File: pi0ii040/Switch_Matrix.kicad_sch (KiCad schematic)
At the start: 1 part

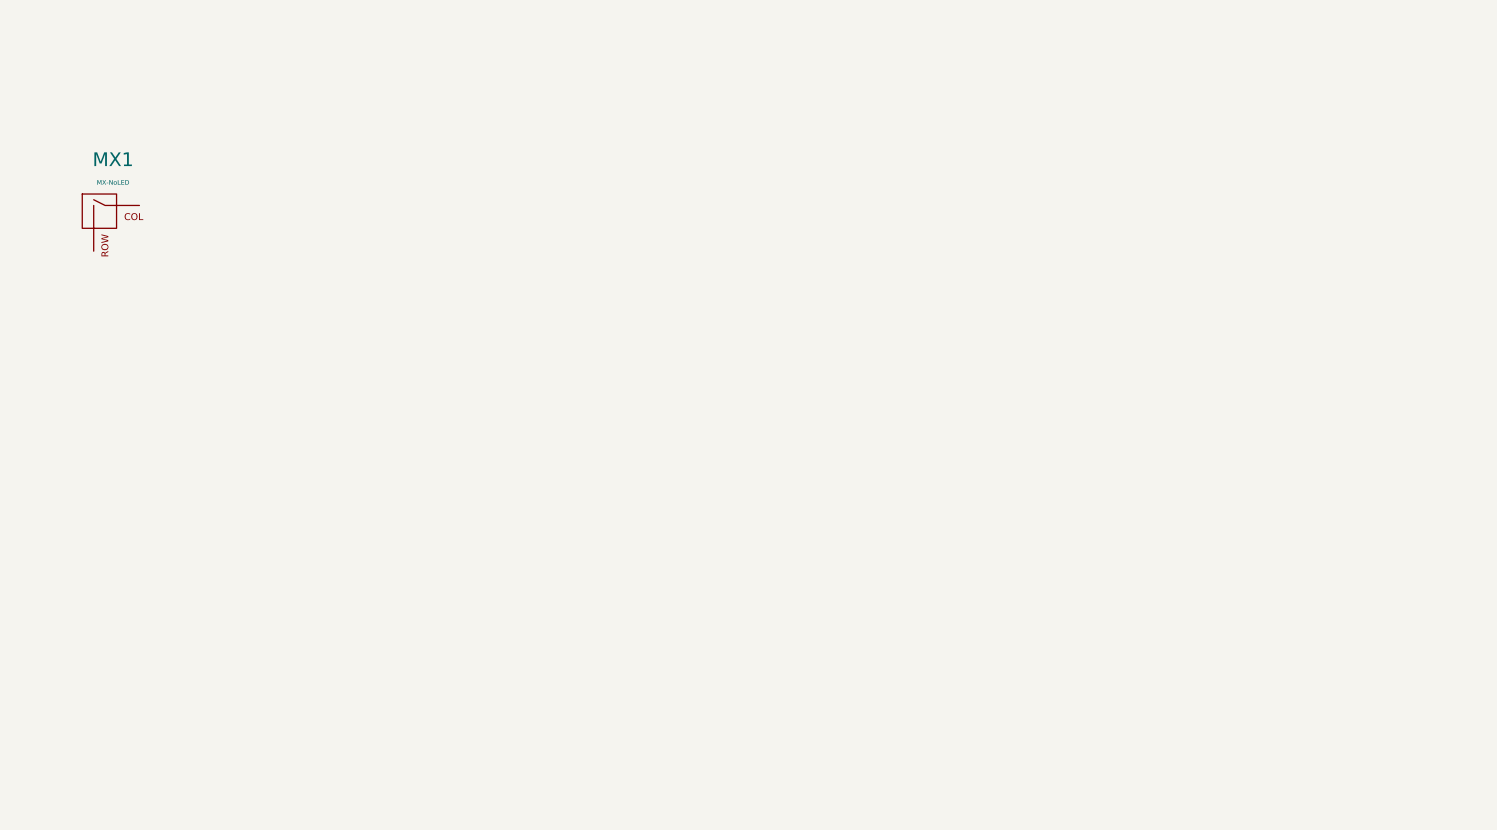
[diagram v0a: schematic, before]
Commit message: Finish? pcb
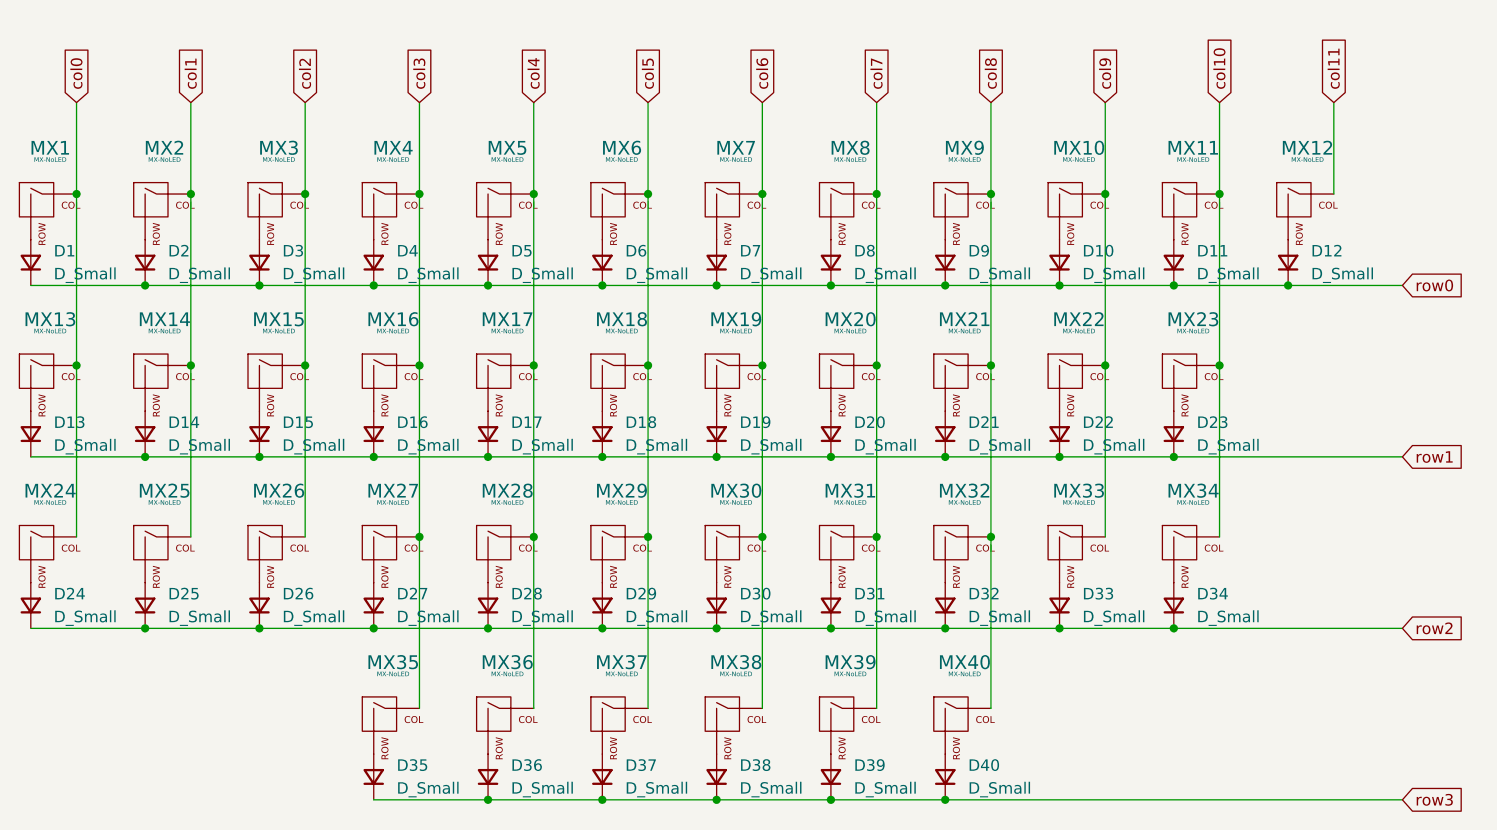
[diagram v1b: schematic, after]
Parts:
- removed MX1: MX-NoLED, symbol MX_Alps_Hybrid:MX-NoLED
- added D1, D10, D11, D12, D13, D14, D15, D16, D17, D18, D19, D2, D20, D21, D22, D23, D24, D25, D26, D27, D28, D29, D3, D30, D31, D32, D33, D34, D35, D36, D37, D38, D39, D4, D40, D5, D6, D7, D8, D9: D_Small, Diode_SMD:D_SOD-123, symbol Device:D_Small
- added MX1, MX10, MX11, MX12, MX14, MX15, MX16, MX17, MX18, MX19, MX2, MX20, MX21, MX22, MX25, MX26, MX27, MX28, MX29, MX3, MX30, MX31, MX32, MX33, MX35, MX4, MX40, MX5, MX6, MX7, MX8, MX9: MX-NoLED, MX_Only:MXOnly-1U-NoLED, symbol cipulot_parts:MX-NoLED
- added MX13, MX34, MX36, MX39: MX-NoLED, MX_Only:MXOnly-1.25U-NoLED, symbol cipulot_parts:MX-NoLED
- added MX23, MX24: MX-NoLED, MX_Only:MXOnly-1.75U-NoLED, symbol cipulot_parts:MX-NoLED
- added MX37: MX-NoLED, MX_Only:MXOnly-2.75U-ReversedStabilizers-NoLED, symbol cipulot_parts:MX-NoLED
- added MX38: MX-NoLED, MX_Only:MXOnly-2.25U-ReversedStabilizers-NoLED, symbol cipulot_parts:MX-NoLED
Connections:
- new net: D21.2 (A), MX21.2 (ROW)
- new net: D10.2 (A), MX10.2 (ROW)
- new net: D40.2 (A), MX40.2 (ROW)
- new net: D16.2 (A), MX16.2 (ROW)
- new net: D28.2 (A), MX28.2 (ROW)
- new net: D39.2 (A), MX39.2 (ROW)
- new net: D23.2 (A), MX23.2 (ROW)
- new net: D1.2 (A), MX1.2 (ROW)
- new net: D27.2 (A), MX27.2 (ROW)
- new net: D32.2 (A), MX32.2 (ROW)
- new net: D31.2 (A), MX31.2 (ROW)
- new net: D13.2 (A), MX13.2 (ROW)
- new net: D11.2 (A), MX11.2 (ROW)
- new net: D18.2 (A), MX18.2 (ROW)
- new net: D25.2 (A), MX25.2 (ROW)
- new net: D14.2 (A), MX14.2 (ROW)
- new net: D8.2 (A), MX8.2 (ROW)
- new net: D22.2 (A), MX22.2 (ROW)
- new net: D26.2 (A), MX26.2 (ROW)
- new net: D34.2 (A), MX34.2 (ROW)
- new net: D19.2 (A), MX19.2 (ROW)
- new net: D12.2 (A), MX12.2 (ROW)
- new net: D15.2 (A), MX15.2 (ROW)
- new net: D4.2 (A), MX4.2 (ROW)
- new net: D5.2 (A), MX5.2 (ROW)
- new net: D24.2 (A), MX24.2 (ROW)
- new net: D30.2 (A), MX30.2 (ROW)
- new net: D37.2 (A), MX37.2 (ROW)
- new net: D17.2 (A), MX17.2 (ROW)
- new net: D35.2 (A), MX35.2 (ROW)
- new net: D20.2 (A), MX20.2 (ROW)
- new net: D3.2 (A), MX3.2 (ROW)
- new net: D6.2 (A), MX6.2 (ROW)
- new net: D38.2 (A), MX38.2 (ROW)
- new net: D29.2 (A), MX29.2 (ROW)
- new net: D2.2 (A), MX2.2 (ROW)
- new net: D33.2 (A), MX33.2 (ROW)
- new net: D9.2 (A), MX9.2 (ROW)
- new net: D7.2 (A), MX7.2 (ROW)
- new net: D36.2 (A), MX36.2 (ROW)
- new net col0: MX1.1 (COL), MX13.1 (COL), MX24.1 (COL)
- new net col1: MX14.1 (COL), MX2.1 (COL), MX25.1 (COL)
- new net col10: MX11.1 (COL), MX23.1 (COL), MX34.1 (COL)
- new net col11: MX12.1 (COL)
- new net col2: MX15.1 (COL), MX26.1 (COL), MX3.1 (COL)
- new net col3: MX16.1 (COL), MX27.1 (COL), MX35.1 (COL), MX4.1 (COL)
- new net col4: MX17.1 (COL), MX28.1 (COL), MX36.1 (COL), MX5.1 (COL)
- new net col5: MX18.1 (COL), MX29.1 (COL), MX37.1 (COL), MX6.1 (COL)
- new net col6: MX19.1 (COL), MX30.1 (COL), MX38.1 (COL), MX7.1 (COL)
- new net col7: MX20.1 (COL), MX31.1 (COL), MX39.1 (COL), MX8.1 (COL)
- new net col8: MX21.1 (COL), MX32.1 (COL), MX40.1 (COL), MX9.1 (COL)
- new net col9: MX10.1 (COL), MX22.1 (COL), MX33.1 (COL)
- new net row0: D1.1 (K), D10.1 (K), D11.1 (K), D12.1 (K), D2.1 (K), D3.1 (K), D4.1 (K), D5.1 (K), D6.1 (K), D7.1 (K), D8.1 (K), D9.1 (K)
- new net row1: D13.1 (K), D14.1 (K), D15.1 (K), D16.1 (K), D17.1 (K), D18.1 (K), D19.1 (K), D20.1 (K), D21.1 (K), D22.1 (K), D23.1 (K)
- new net row2: D24.1 (K), D25.1 (K), D26.1 (K), D27.1 (K), D28.1 (K), D29.1 (K), D30.1 (K), D31.1 (K), D32.1 (K), D33.1 (K), D34.1 (K)
- new net row3: D35.1 (K), D36.1 (K), D37.1 (K), D38.1 (K), D39.1 (K), D40.1 (K)
